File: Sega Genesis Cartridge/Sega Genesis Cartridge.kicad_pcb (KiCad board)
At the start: 2 copper layers, 7 parts, among them J1 edge_connector, SW1 my_SW_SP3T, U1 my_SST39SF040, U2 my_SST39SF040

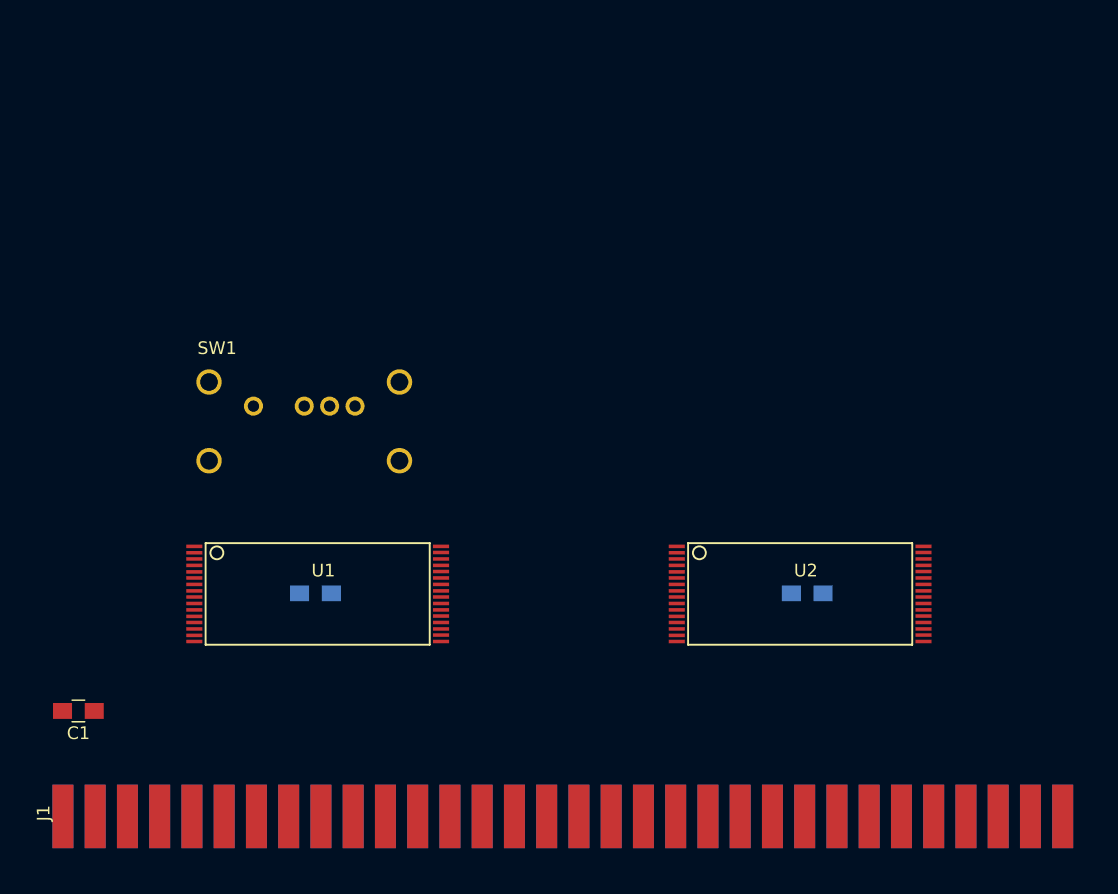
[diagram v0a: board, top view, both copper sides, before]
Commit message: PCB layout
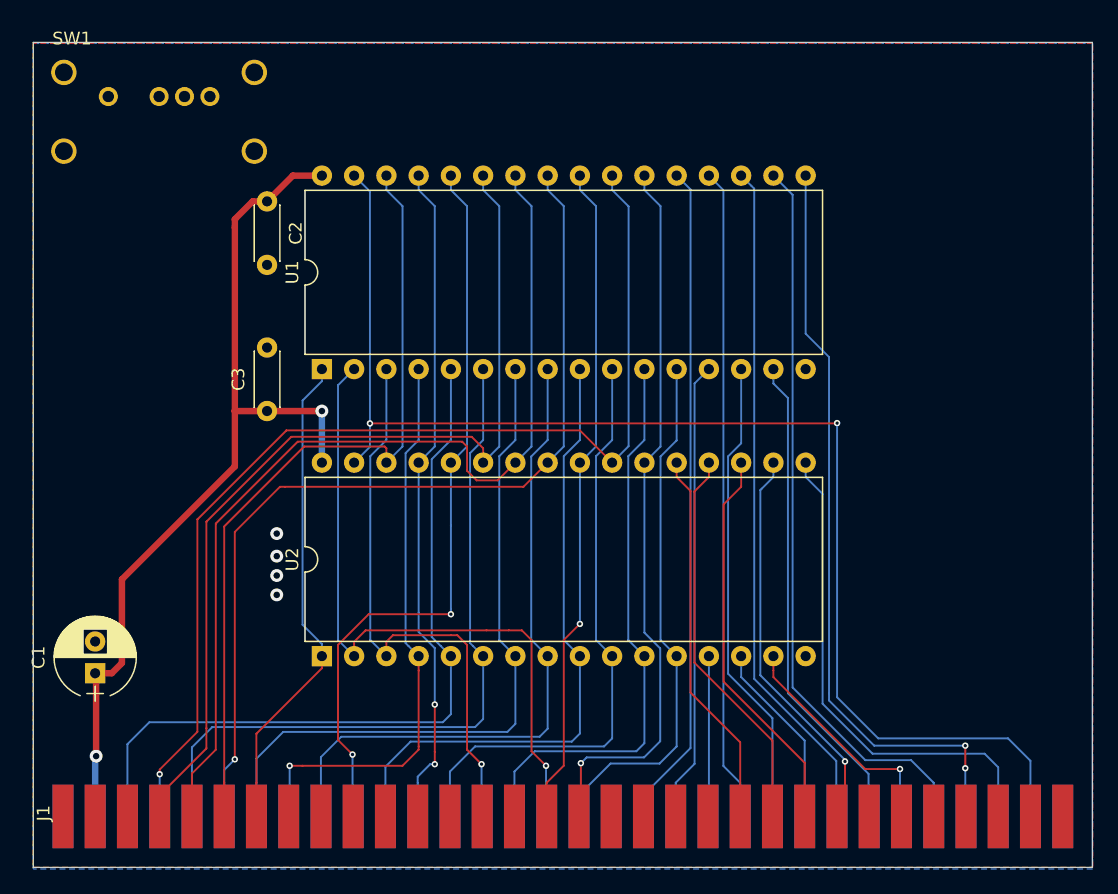
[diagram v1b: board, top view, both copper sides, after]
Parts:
- C1: footprint Capacitors_SMD:C_0805_HandSoldering -> Capacitors_ThroughHole:CP_Radial_D6.3mm_P2.50mm
- C2, C3: footprint Capacitors_SMD:C_0805_HandSoldering -> Capacitors_ThroughHole:C_Disc_D4.3mm_W1.9mm_P5.00mm; moved to F.Cu
- U1, U2: footprint SMD_Packages:TSOP32SP -> Package_DIP:DIP-32_W15.24mm
- moved C3 44.9 mm to (116.1, 65.5), turned to 90 degrees
- moved U2 37.9 mm to (120.4, 84.8), turned to 90 degrees
- moved C2 31.1 mm to (116.1, 49.0), turned to 270 degrees
- moved SW1 26.9 mm to (100.1, 38.9)
- moved U1 17.8 mm to (120.4, 62.2), turned to 90 degrees
- moved C1 3.25 mm to (102.5, 86.2), turned to 90 degrees
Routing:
- net /~WE: track 0.00 -> 103.8 mm, vias 0 -> 2
- net /A11: track 0.00 -> 84.9 mm, vias 0 -> 1
- net /A10: track 0.00 -> 76.7 mm
- net /A9: track 0.00 -> 74.5 mm
- net /A12: track 0.00 -> 73.3 mm, vias 0 -> 1
- net VCC: track 0.00 -> 71.6 mm, vias 0 -> 2
- net /A18: track 0.00 -> 65.7 mm
- net /A8: track 0.00 -> 60.6 mm
- net /D3: track 0.00 -> 59.9 mm, vias 0 -> 2
- net /A14: track 0.00 -> 59.5 mm, vias 0 -> 2
- net /D4: track 0.00 -> 58.0 mm
- net /A7: track 0.00 -> 57.7 mm
- net /~CE: track 0.00 -> 57.3 mm, vias 0 -> 1
- net /A6: track 0.00 -> 55.1 mm
- net /A17: track 0.00 -> 53.8 mm, vias 0 -> 1
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- added copper zone on B.Cu, net GND
- added copper zone on F.Cu, net GND
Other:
- board outline added: 83.4 x 65 mm
- net class Default: clearance 0.2 -> 0.1524; trace_width 0.25 -> 0.1524; via_dia 0.8 -> 0.6858; via_drill 0.4 -> 0.3302
- net class Signal added: clearance 0.1524, trace_width 0.1524, via_dia 0.508, via_drill 0.254
- rule trace_clearance: 0.2 -> 0.1524
- rule trace_min: 0.2 -> 0.1524
- rule via_min_drill: 0.3 -> 0.254
- rule via_min_size: 0.4 -> 0.508
